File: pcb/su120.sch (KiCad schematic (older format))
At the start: 134 parts, among them J1 MJ-4PP-9, J2 Conn_01x03, J3 Conn_01x08, J4 Conn_01x08, J5 Conn_01x03, J6 MJ-4PP-9, SW1 SW_Push, SW10 SW_Push, SW11 SW_Push, SW12 SW_Push, SW13 SW_Push, SW14 SW_Push, SW15 SW_Push, SW16 SW_Push, SW17 SW_Push, SW18 SW_Push, SW19 SW_Push, SW2 SW_Push, SW20 SW_Push, SW21 SW_Push, SW3 SW_Push, SW4 SW_Push, SW5 SW_Push, SW6 SW_Push, SW7 SW_Push, SW8 SW_Push, SW9 SW_Push, U1 ProMicro

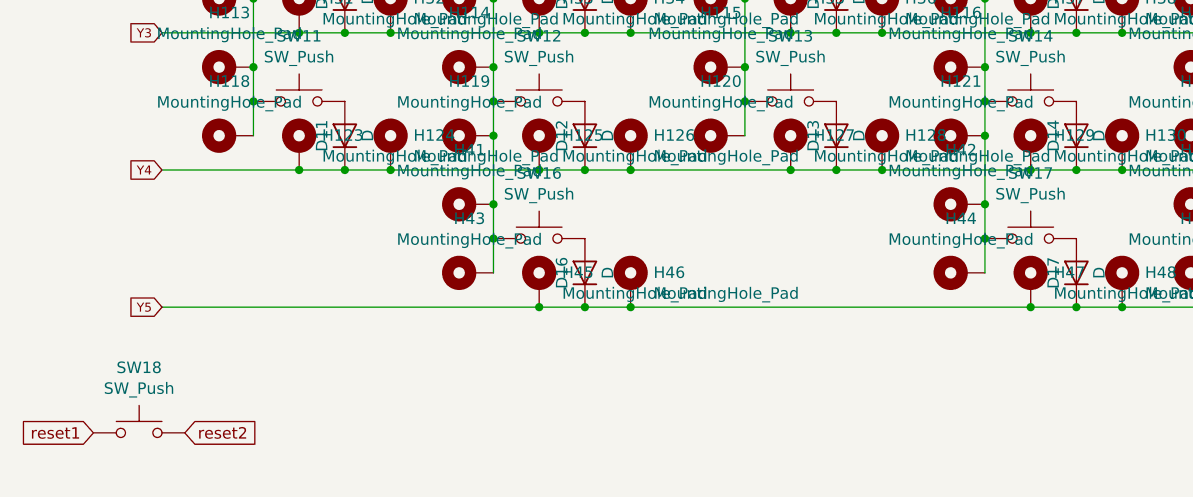
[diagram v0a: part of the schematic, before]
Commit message: rev5
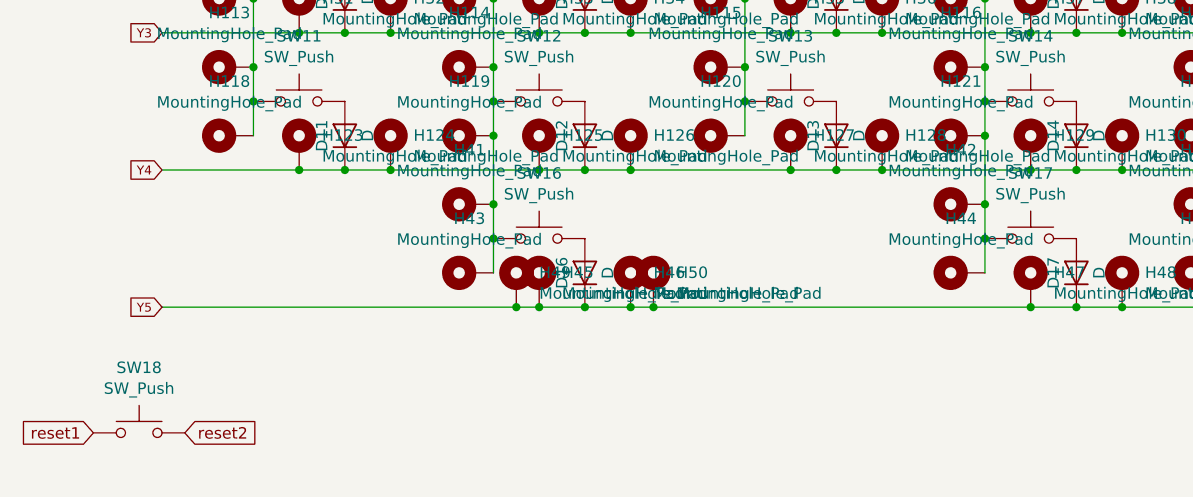
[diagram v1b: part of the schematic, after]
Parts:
- added H49, H50: MountingHole_Pad, #footprint:1pin_conn, symbol Mechanical:MountingHole_Pad
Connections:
- net Y5: now also H49.1, H50.1
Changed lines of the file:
@@
 Title "SU120 Yakitori Keyboard"
 Date ""
-Rev "4"
+Rev "5"
 Comp "@e3w2q"
 Comment1 ""
@@
 Connection ~ 10250 3150
 Wire Wire Line
-	7650 3900 9400 3900
-Wire Wire Line
-	5600 3900 7250 3900
+	7650 3900 7750 3900
+Wire Wire Line
+	5600 3900 7150 3900
 Wire Wire Line
 	5600 3300 6200 3300
@@
 Wire Wire Line
 	6000 800  6000 1650
+$Comp
+L Mechanical:MountingHole_Pad H50
+U 1 1 5D363A98
+P 7750 3800
+F 0 "H50" H 7850 3851 50  0000 L CNN
+F 1 "MountingHole_Pad" H 7850 3760 50  0000 L CNN
+F 2 "#footprint:1pin_conn" H 7750 3800 50  0001 C CNN
+F 3 "~" H 7750 3800 50  0001 C CNN
+	1    7750 3800
+	1    0    0    -1
+$EndComp
+Connection ~ 7750 3900
+Wire Wire Line
+	7750 3900 9400 3900
+$Comp
+L Mechanical:MountingHole_Pad H49
+U 1 1 5D363BD2
+P 7150 3800
+F 0 "H49" H 7250 3851 50  0000 L CNN
+F 1 "MountingHole_Pad" H 7250 3760 50  0000 L CNN
+F 2 "#footprint:1pin_conn" H 7150 3800 50  0001 C CNN
+F 3 "~" H 7150 3800 50  0001 C CNN
+	1    7150 3800
+	1    0    0    -1
+$EndComp
+Connection ~ 7150 3900
+Wire Wire Line
+	7150 3900 7250 3900
 $EndSCHEMATC

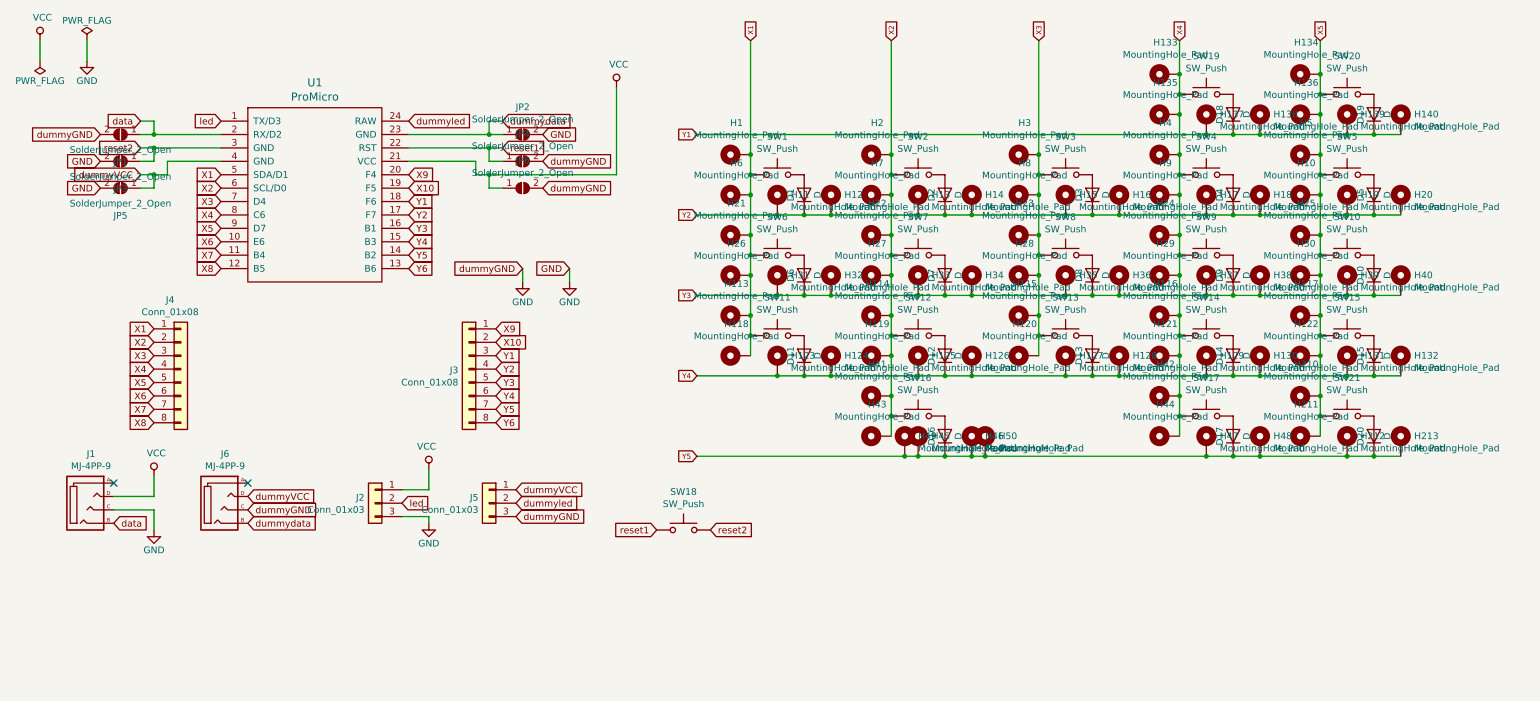
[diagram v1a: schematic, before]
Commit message: Rev6
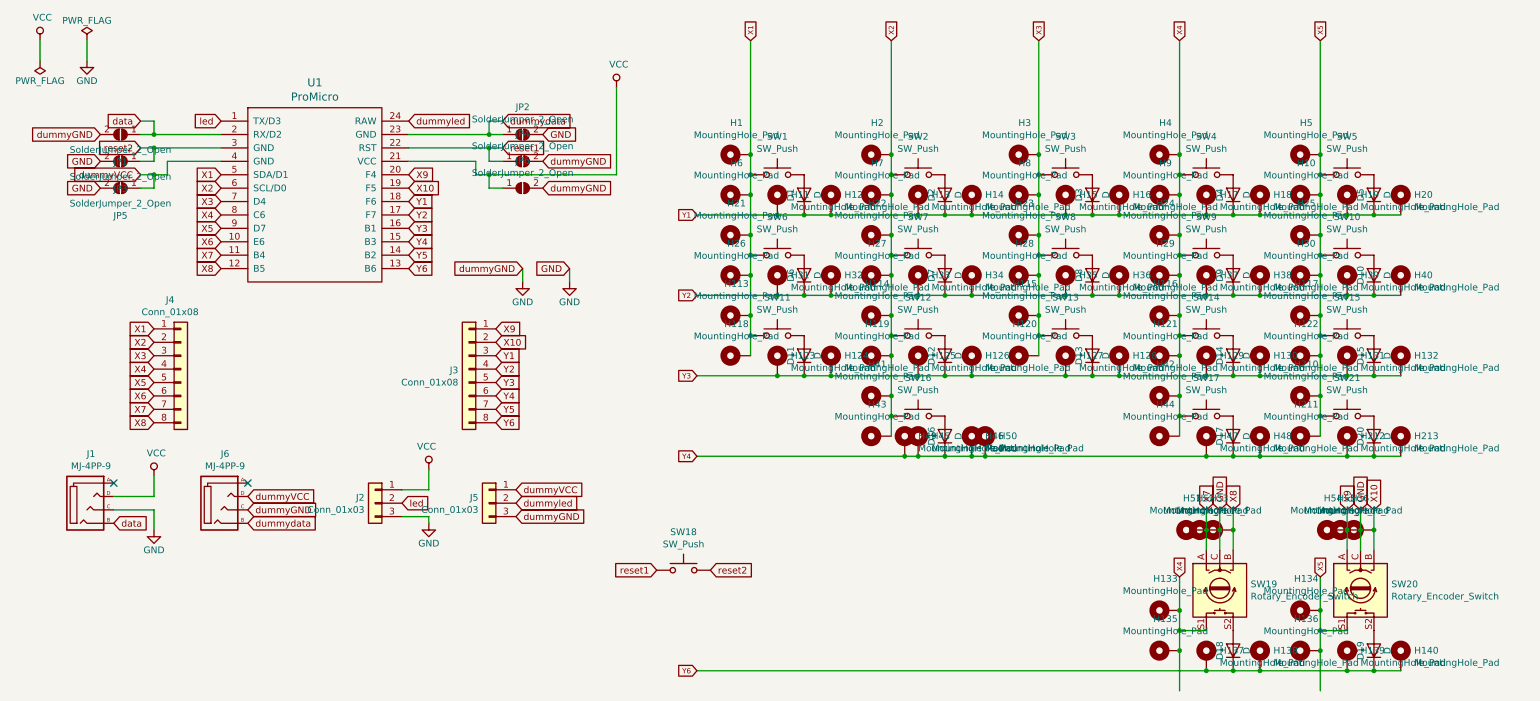
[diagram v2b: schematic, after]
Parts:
- removed SW19, SW20: SW_Push, #footprint:CherryMX_Choc_Hotswap_rev4, symbol Switch:SW_Push
- added H51, H52, H53, H54, H55, H56: MountingHole_Pad, #footprint:1pin_conn, symbol Mechanical:MountingHole_Pad
- added SW19, SW20: Rotary_Encoder_Switch, #footprint:RotaryEncoder_Alps_EC11E-Switch_Vertical_H20mm_rev2, symbol Device:Rotary_Encoder_Switch
- SW1, SW10, SW11, SW12, SW13, SW14, SW15, SW16, SW17, SW2, SW3, SW4, SW5, SW6, SW7, SW8, SW9: footprint #footprint:CherryMX_Choc_Hotswap_rev4 -> #footprint:CherryMX_MidHeight_Choc_Hotswap_rev5
- U1: footprint #footprint:ArduinoProMicro-ZigZag_rev4 -> #footprint:ArduinoProMicro-ZigZag_rev5
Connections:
- net GND: now also H52.1, H55.1, SW19.C, SW20.C
- net X10: now also H56.1, SW20.B
- net X4: now also SW19.S1
- net X5: now also SW20.S1
- net X7: now also H51.1, SW19.A
- net X8: now also H53.1, SW19.B
- net X9: now also H54.1, SW20.A
- net Y1: now also D1.1 (K), D2.1 (K), D3.1 (K), D4.1 (K), D5.1 (K), H11.1, H12.1, H13.1, H14.1, H15.1, H16.1, H17.1, H18.1, H19.1, H20.1; no longer D18.1 (K), D19.1 (K), H137.1, H138.1, H139.1, H140.1
- net Y2: now also D10.1 (K), D6.1 (K), D7.1 (K), D8.1 (K), D9.1 (K), H31.1, H32.1, H33.1, H34.1, H35.1, H36.1, H37.1, H38.1, H39.1, H40.1; no longer D1.1 (K), D2.1 (K), D3.1 (K), D4.1 (K), D5.1 (K), H11.1, H12.1, H13.1, H14.1, H15.1, H16.1, H17.1, H18.1, H19.1, H20.1
- net Y3: now also D11.1 (K), D12.1 (K), D13.1 (K), D14.1 (K), D15.1 (K), H123.1, H124.1, H125.1, H126.1, H127.1, H128.1, H129.1, H130.1, H131.1, H132.1; no longer D10.1 (K), D6.1 (K), D7.1 (K), D8.1 (K), D9.1 (K), H31.1, H32.1, H33.1, H34.1, H35.1, H36.1, H37.1, H38.1, H39.1, H40.1
- net Y4: now also D16.1 (K), D17.1 (K), D20.1 (K), H212.1, H213.1, H45.1, H46.1, H47.1, H48.1, H49.1, H50.1; no longer D11.1 (K), D12.1 (K), D13.1 (K), D14.1 (K), D15.1 (K), H123.1, H124.1, H125.1, H126.1, H127.1, H128.1, H129.1, H130.1, H131.1, H132.1
- net Y5: no longer D16.1 (K), D17.1 (K), D20.1 (K), H212.1, H213.1, H45.1, H46.1, H47.1, H48.1, H49.1, H50.1
- net Y6: now also D18.1 (K), D19.1 (K), H137.1, H138.1, H139.1, H140.1
- net at D18.2 (A): now also SW19.S2
- net at D19.2 (A): now also SW20.S2
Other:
- moved on the sheet: D18, D19, H133, H134, H135, H136, H137, H138, H139, H140, SW18
